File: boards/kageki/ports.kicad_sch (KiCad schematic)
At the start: 13 parts, among them J1 Conn_01x06, J2 Conn_02x10_Top_Bottom, J3 Conn_01x06, J4 Conn_01x06, SW1 SW_DIP_x04

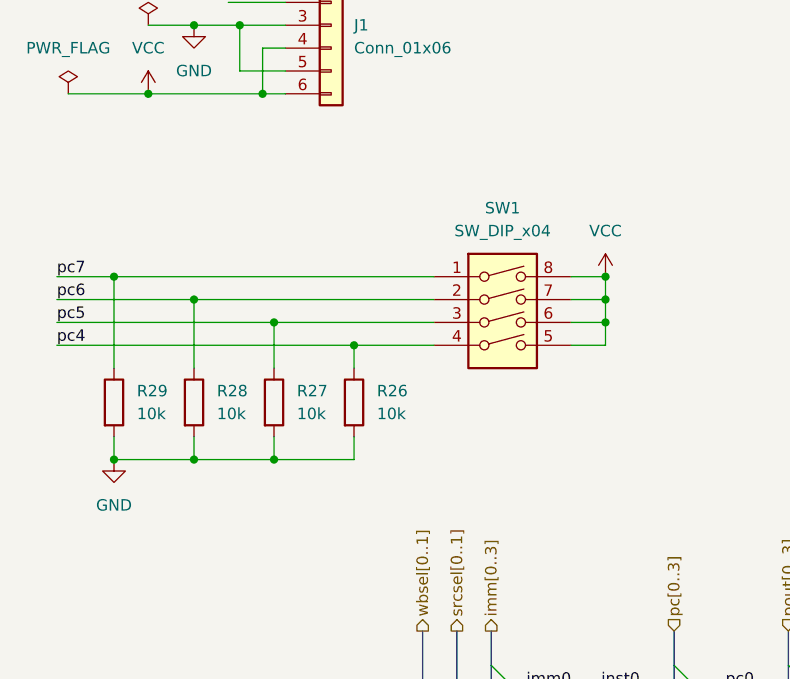
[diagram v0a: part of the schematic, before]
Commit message: kageki: add board design
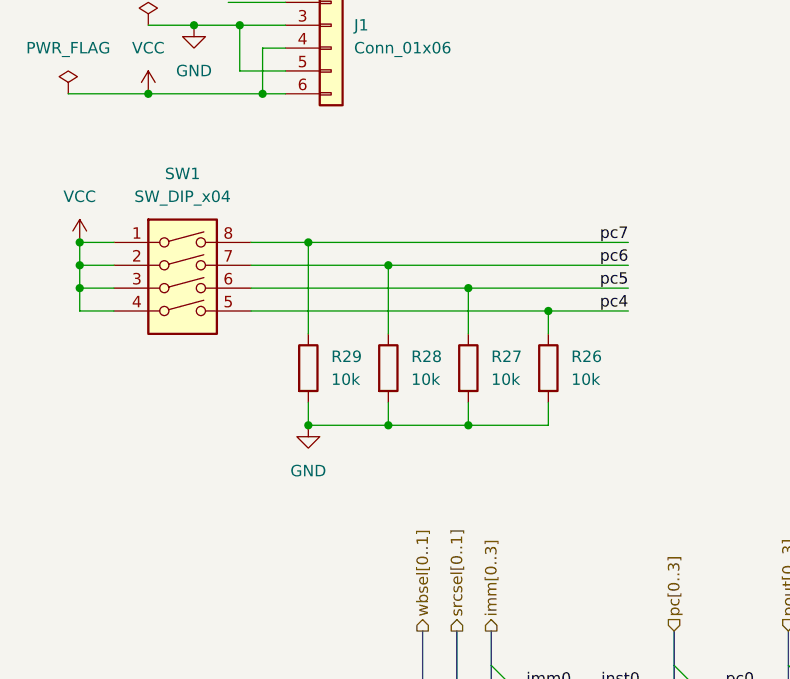
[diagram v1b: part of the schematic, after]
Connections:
- net VCC: now also SW1.1, SW1.2, SW1.3, SW1.4; no longer SW1.5, SW1.6, SW1.7, SW1.8
- net pc4: now also SW1.5; no longer SW1.4
- net pc5: now also SW1.6; no longer SW1.3
- net pc6: now also SW1.7; no longer SW1.2
- net pc7: now also SW1.8; no longer SW1.1
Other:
- moved on the sheet: R26, R27, R28, R29, SW1

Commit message: unify libraries
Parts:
- J2: footprint PrjLibrary_CalicoCPU:PinHeader_2x10_P2.54mm_Vertical_Top_Bottom -> ModifiedKiCadLibrary:PinHeader_2x10_P2.54mm_Vertical_Top_Bottom
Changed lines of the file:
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@@
     (property "Reference" "J2" (id 0) (at 73.66 25.4 0))
     (property "Value" "Conn_02x10_Top_Bottom" (id 1) (at 73.66 27.94 0))
-    (property "Footprint" "PrjLibrary_CalicoCPU:PinHeader_2x10_P2.54mm_Vertical_Top_Bottom" (id 2) (at 72.39 41.91 0)
+    (property "Footprint" "ModifiedKiCadLibrary:PinHeader_2x10_P2.54mm_Vertical_Top_Bottom" (id 2) (at 72.39 41.91 0)
       (effects (font (size 1.27 1.27)) hide)
     )
